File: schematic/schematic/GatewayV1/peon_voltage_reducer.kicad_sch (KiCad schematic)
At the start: 20 parts, among them Q4 BSS138, U10 LMV358

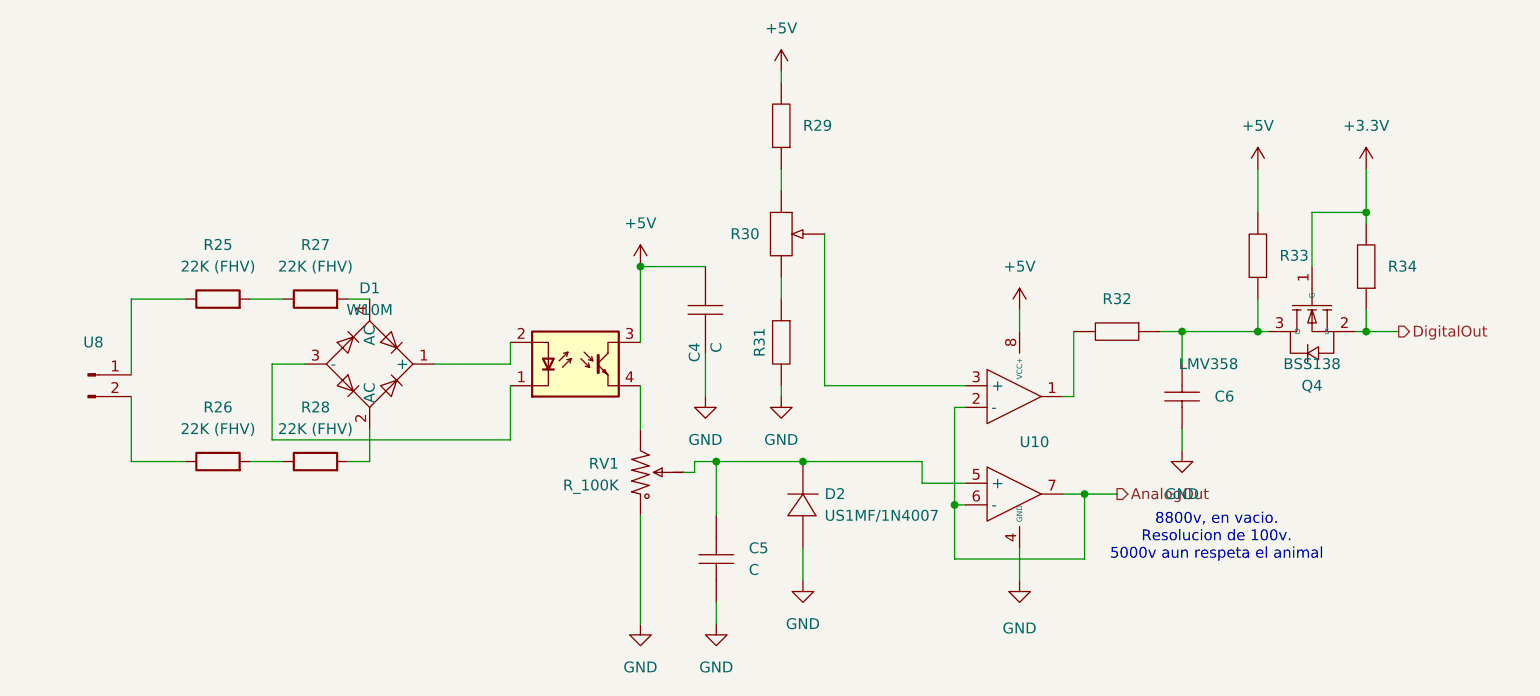
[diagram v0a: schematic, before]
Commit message: Feat Board Completed, in production
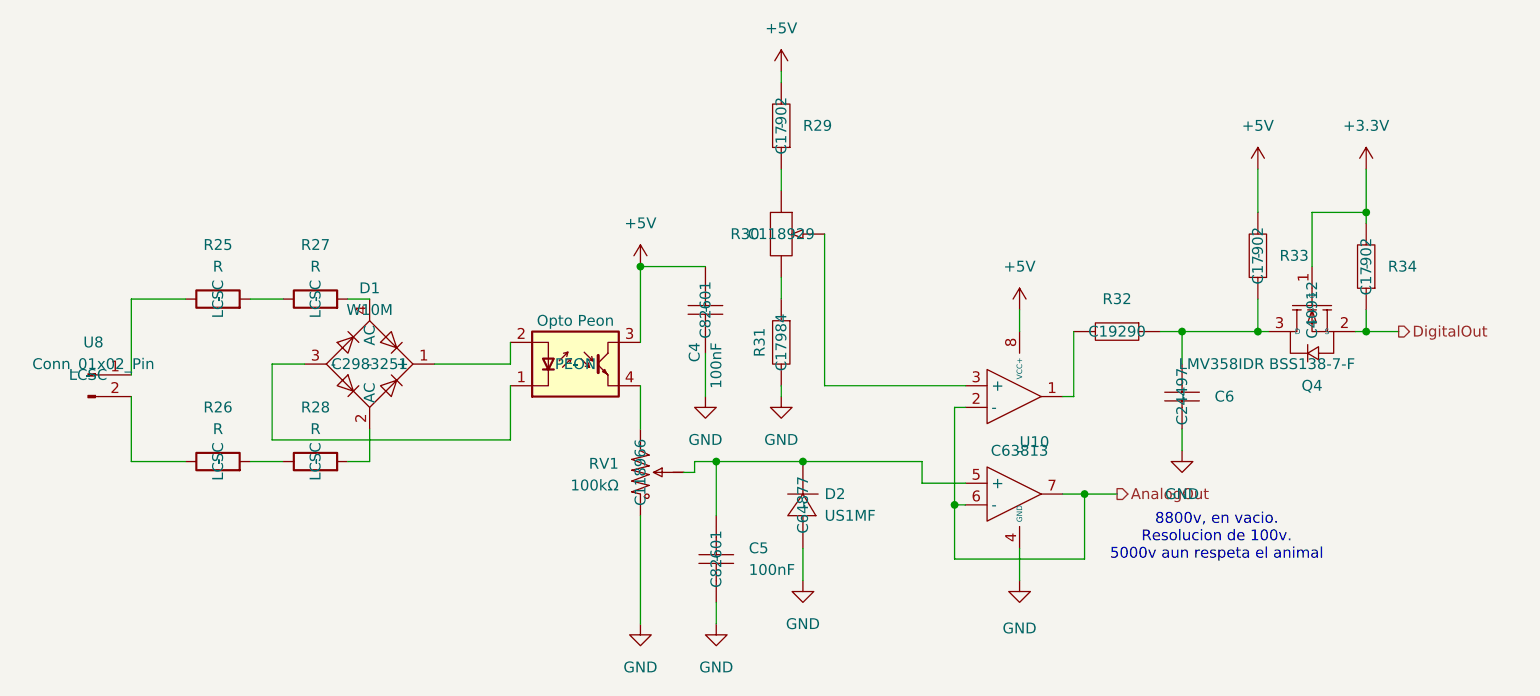
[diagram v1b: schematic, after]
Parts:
- C4, C5: value C -> 100nF; Comments (none) -> -; JLCPCB Part (none) -> C82601; LCSC (none) -> C82601
- C6: Comments (none) -> -; JLCPCB Part (none) -> C24497; LCSC (none) -> C24497
- D1: Comments (none) -> -; JLCPCB Part (none) -> C2983251; LCSC (none) -> C2983251
- D2: value US1MF/1N4007 -> US1MF; Comments (none) -> -; JLCPCB Part (none) -> C64877; LCSC (none) -> C64877
- Q4: value BSS138 -> BSS138-7-F; Comments (none) -> -; JLCPCB Part (none) -> C40912; LCSC (none) -> C40912
- R25, R26, R27, R28: value 22K (FHV) -> R; JLCPCB Part (none) -> -; LCSC (none) -> -; Part No FVR01B -> (none); Supplier (none) -> LCSC; Supplier Part (none) -> -
- R29, R33, R34: Comments (none) -> -; JLCPCB Part (none) -> C17902; LCSC (none) -> C17902
- R30: value 2kΩ/2.2K -> 2kΩ; JLCPCB Part (none) -> C118929; LCSC (none) -> C118929
- R31: JLCPCB Part (none) -> C17984; LCSC (none) -> C17984
- R32: JLCPCB Part (none) -> C19290; LCSC (none) -> C19290
- RV1: value R_100K -> 100kΩ; JLCPCB Part (none) -> C118966; LCSC (none) -> C118966
- U10: value LMV358 -> LMV358IDR; Comments (none) -> -; JLCPCB Part (none) -> C63813; LCSC (none) -> C63813
- U8: value ~ -> Conn_01x02_Pin; JLCPCB Part (none) -> -; LCSC (none) -> -; Supplier (none) -> LCSC; Supplier Part (none) -> -
- U9: value ~ -> Opto Peon; Comentarios (none) -> -; JLCPCB Part (none) -> -; LCSC (none) -> -; Supplier (none) -> PEON; Supplier Part (none) -> -
